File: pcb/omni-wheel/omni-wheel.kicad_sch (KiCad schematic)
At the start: 12 parts, among them J1 Motor1_input, J2 Motor2_input, J3 Motor4_input, J4 Motor3_input, J5 STLINK, J6 3.3V Input, J7 12V Input, U1 SN754410NE, U2 SN754410NE, U3 STM32F030R8Tx

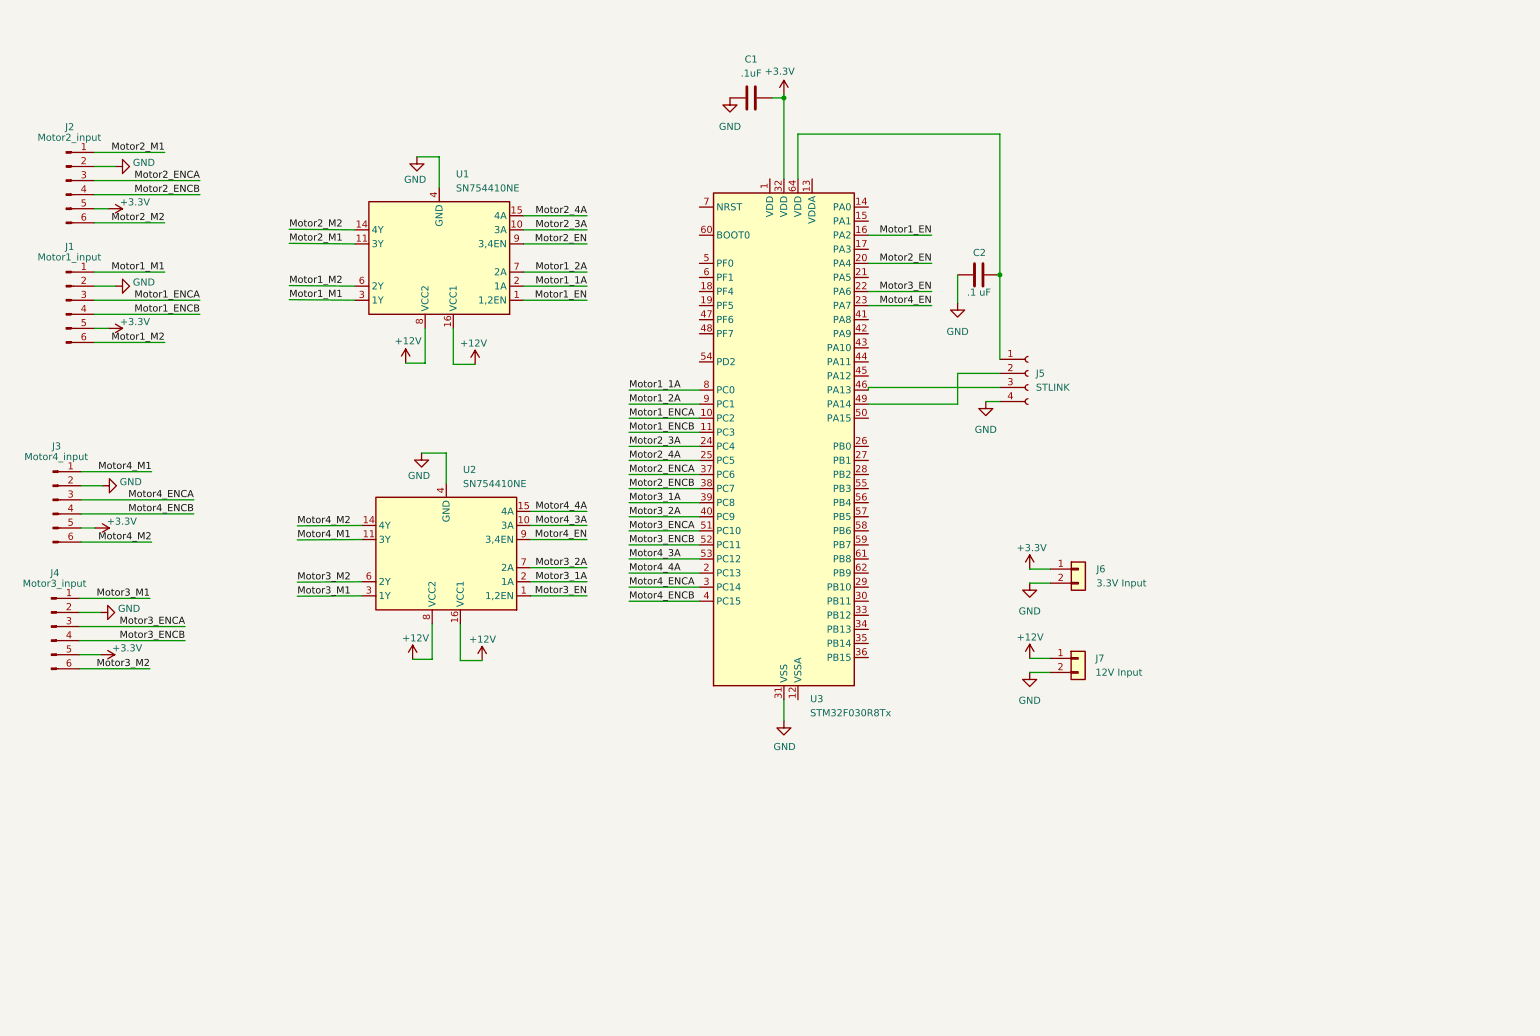
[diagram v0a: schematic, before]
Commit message: PCB save
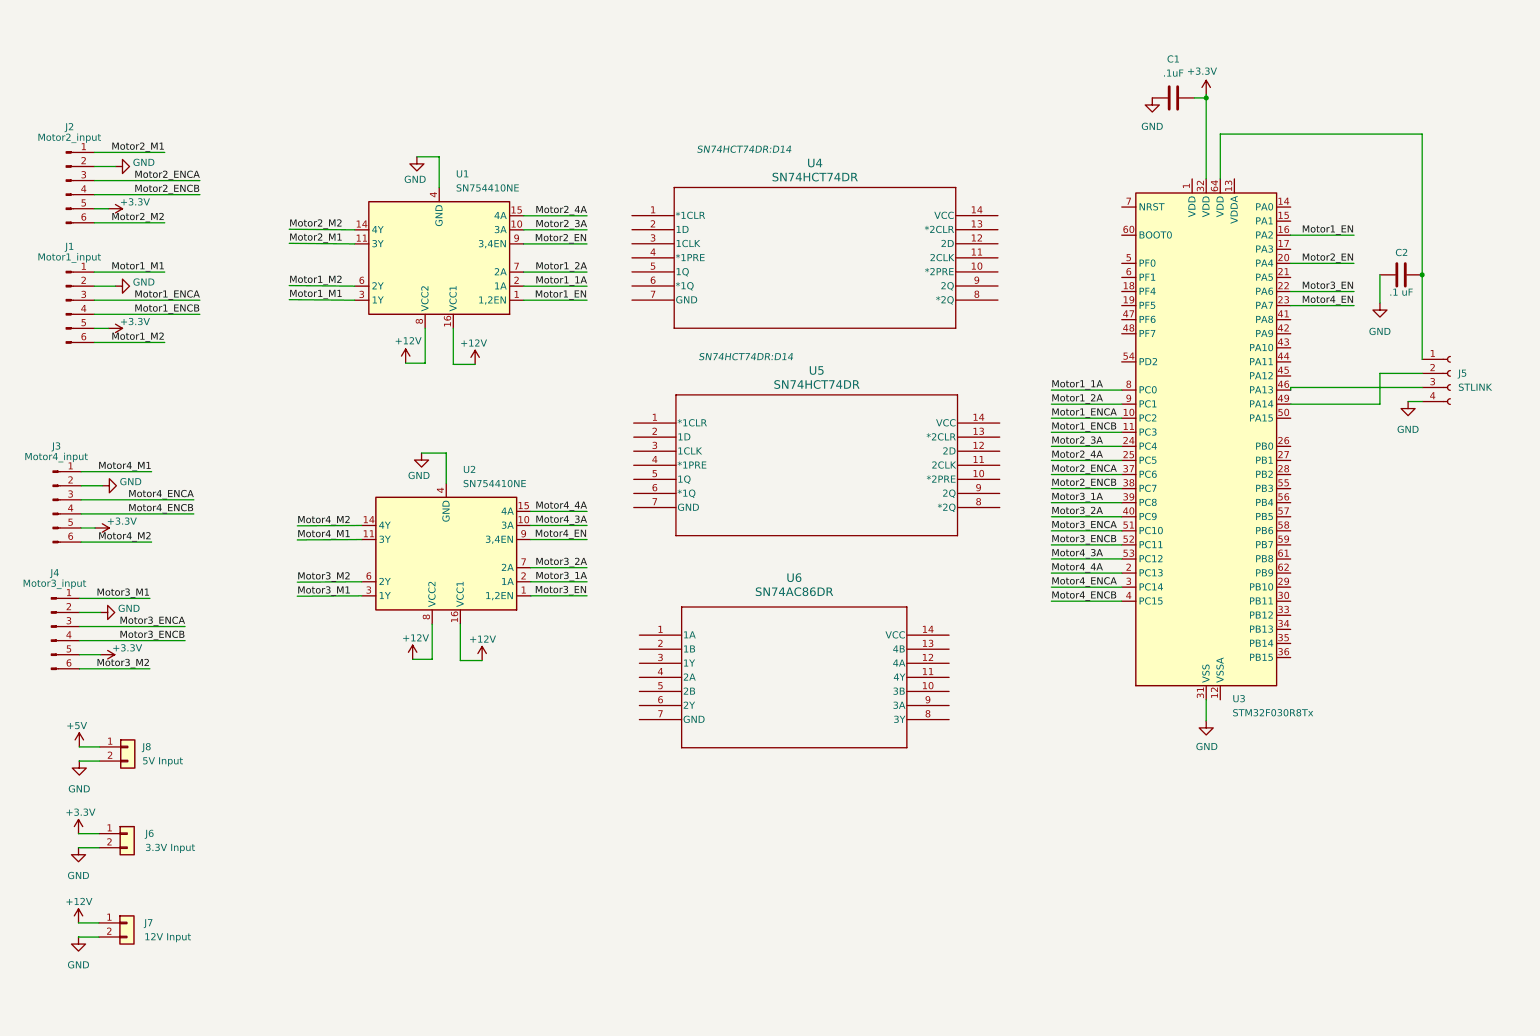
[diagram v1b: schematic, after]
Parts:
- added J8: 5V Input, symbol Connector_Generic:Conn_01x02
- added U4, U5: SN74HCT74DR, SN74HCT74DR:D14, symbol SN74HCT74DR:SN74HCT74DR
- added U6: SN74AC86DR, D14, symbol SN74AC86DR:SN74AC86DR
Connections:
- net GND: now also J8.2 (Pin_2)
- new net +5V: J8.1 (Pin_1)
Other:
- moved on the sheet: C1, C2, J5, J6, J7, U3

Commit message: pcb update for home
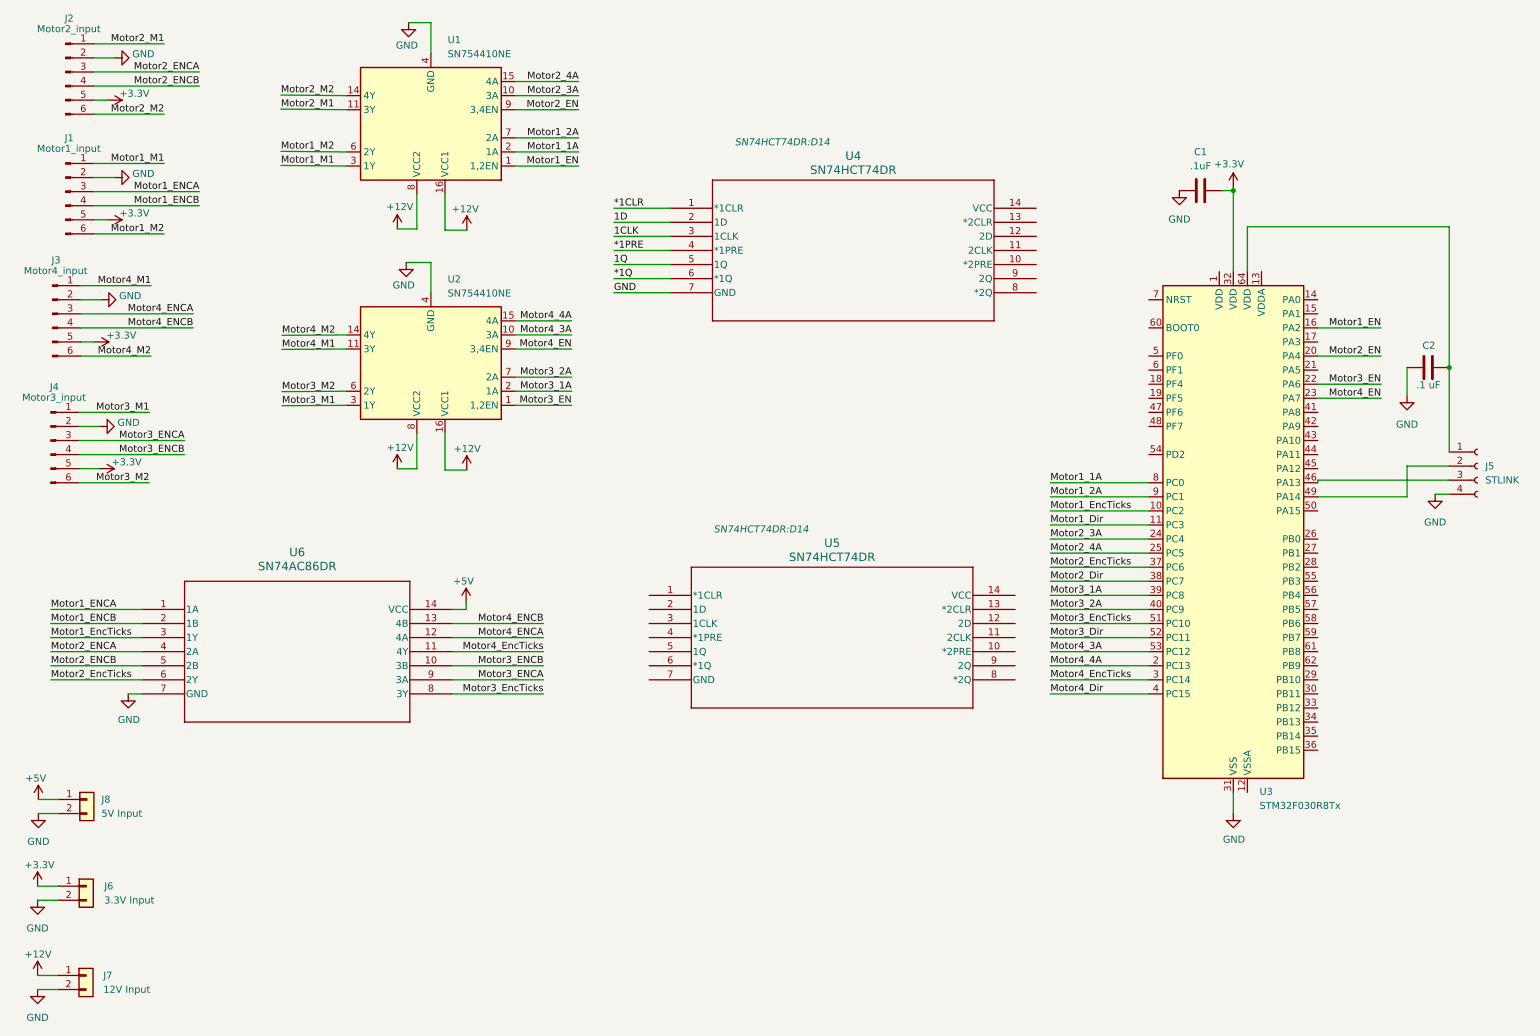
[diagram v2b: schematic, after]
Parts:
- J6, J7, J8: footprint (none) -> Connector_AMASS:AMASS_XT60PW-M_1x02_P7.20mm_Horizontal
- U6: footprint D14 -> SN74AC86DR:D14
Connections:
- net +5V: now also U6.14 (VCC)
- net GND: now also U4.7 (GND), U6.7 (GND)
- net Motor1_ENCA: now also U6.1 (1A); no longer U3.10 (PC2)
- net Motor1_ENCB: now also U6.2 (1B); no longer U3.11 (PC3)
- net Motor2_ENCA: now also U6.4 (2A); no longer U3.37 (PC6)
- net Motor2_ENCB: now also U6.5 (2B); no longer U3.38 (PC7)
- net Motor3_ENCA: now also U6.9 (3A); no longer U3.51 (PC10)
- net Motor3_ENCB: now also U6.10 (3B); no longer U3.52 (PC11)
- net Motor4_ENCA: now also U6.12 (4A); no longer U3.3 (PC14)
- net Motor4_ENCB: now also U6.13 (4B); no longer U3.4 (PC15)
- net Motor4_EncTicks: now reaches U6.11 (4Y)
- net Motor4_EncTicks: now also U3.3 (PC14)
- net Motor1_EncTicks: now reaches U6.3 (1Y)
- net Motor1_EncTicks: now also U3.10 (PC2)
- net Motor2_EncTicks: now reaches U6.6 (2Y)
- net Motor2_EncTicks: now also U3.37 (PC6)
- net Motor3_EncTicks: now reaches U6.8 (3Y)
- net Motor3_EncTicks: now also U3.51 (PC10)
- net *1CLR: now reaches U4.1 (*1CLR)
- net 1D: now reaches U4.2 (1D)
- net 1CLK: now reaches U4.3 (1CLK)
- net *1PRE: now reaches U4.4 (*1PRE)
- net 1Q: now reaches U4.5 (1Q)
- net *1Q: now reaches U4.6 (*1Q)
- new net Motor1_Dir: U3.11 (PC3)
- new net Motor2_Dir: U3.38 (PC7)
- new net Motor3_Dir: U3.52 (PC11)
- new net Motor4_Dir: U3.4 (PC15)
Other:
- moved on the sheet: C1, C2, J1, J2, J3, J4, J5, J6, J7, J8, U1, U2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
